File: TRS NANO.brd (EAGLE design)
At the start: 70.5 x 64.5 mm, 32 parts, among them M1 ARDUINO-NANO-3.0, Q5 BC548, Q6 BC548, Q7 BC548, Q8 BC548, T1 351, T3 351, T41 351, T42 351

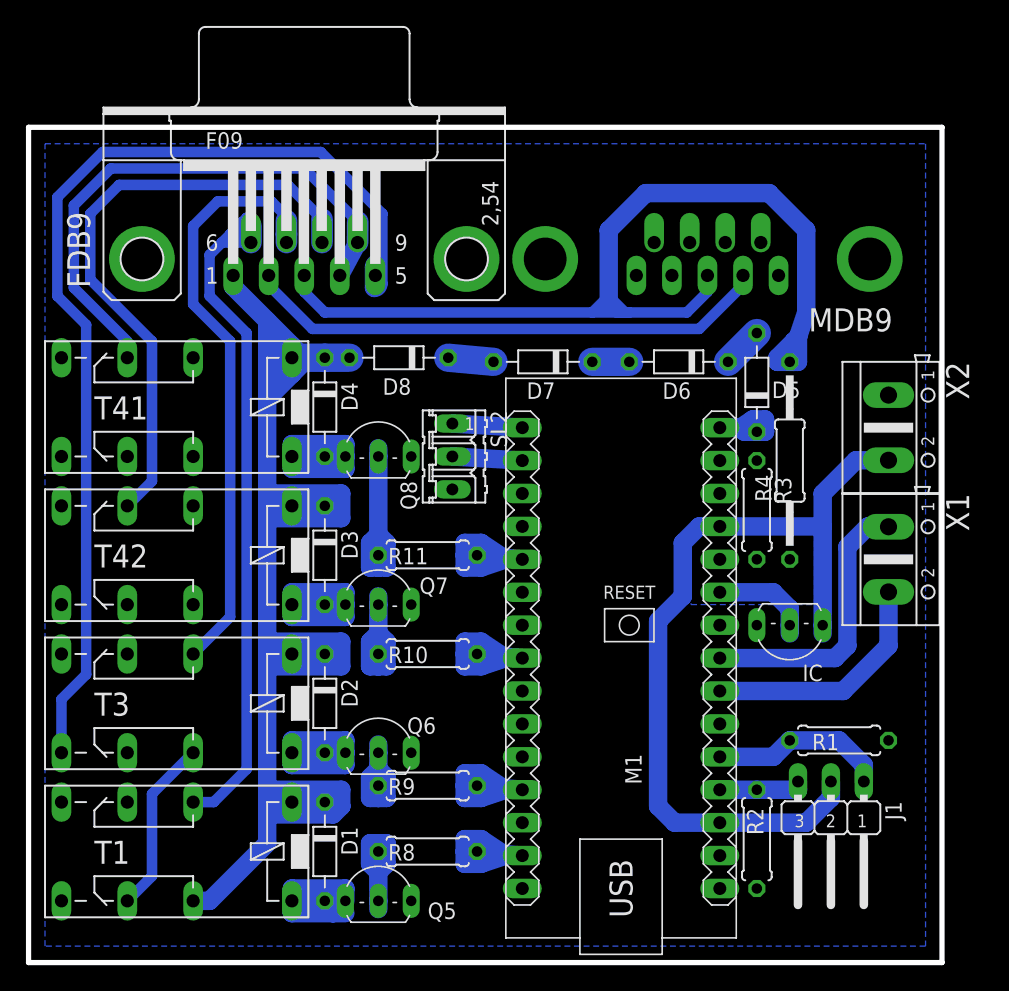
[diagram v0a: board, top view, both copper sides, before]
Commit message: Add
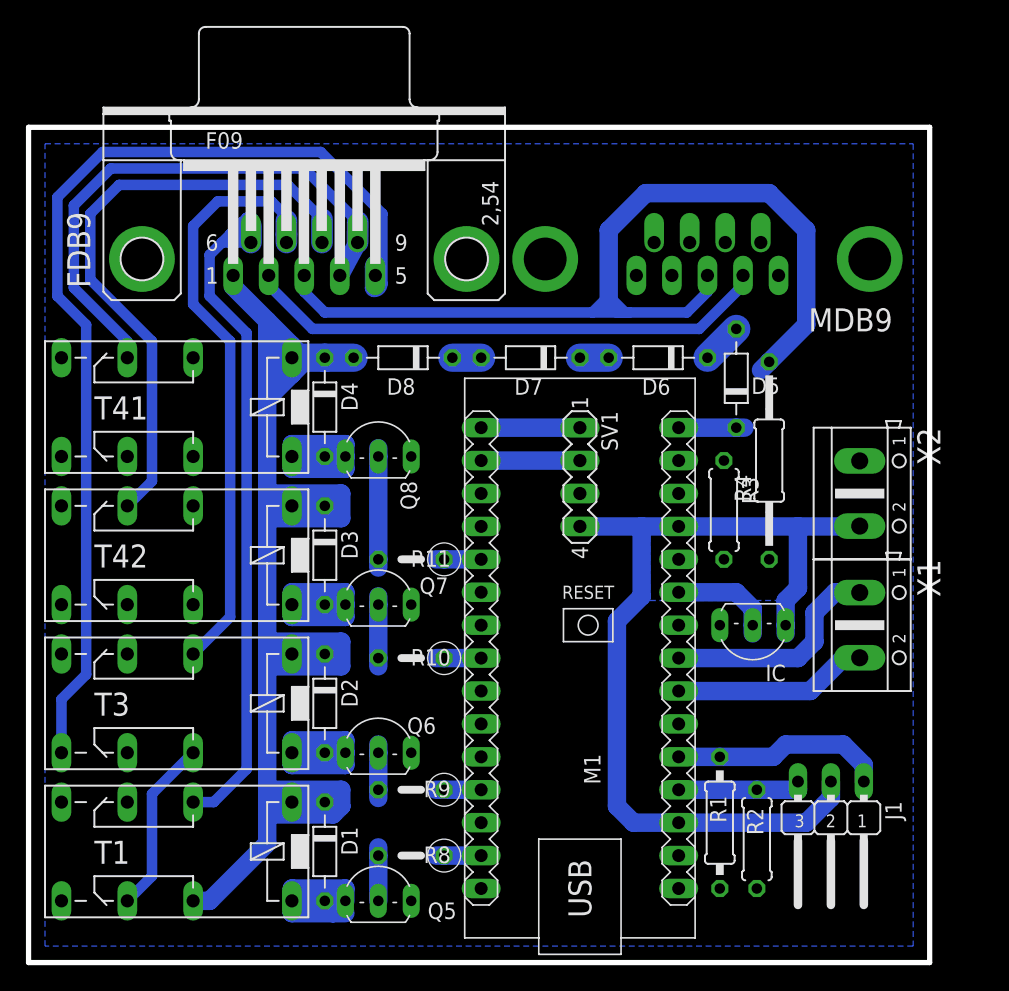
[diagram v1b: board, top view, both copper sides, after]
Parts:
- removed SL2: (no value), con-amp-quick:03P
- added SV1: (no value), con-lstb:MA04-1
- R1: device rcl:0207/7 -> rcl:0207/10
- R10, R11, R8, R9: device rcl:0207/7 -> rcl:0207/5V
- moved R1 11.2 mm to (52.1, 9.53), turned to 90 degrees
- moved X2 5.54 mm to (62.9, 34.9)
- moved X1 5.54 mm to (62.9, 24.8)
- moved M1 3.18 mm to (41.3, 22.2)
- moved IC 2.86 mm to (54.6, 23.5)
- moved R3 2.54 mm to (52.4, 33.7)
- moved D6 1.62 mm to (47.3, 45.4)
- moved D5 1.62 mm to (53.3, 43.8)
- moved R4 1.59 mm to (55.9, 37.5)
- moved R11 1.31 mm to (28.3, 29.8), turned to 180 degrees
- moved R9 1.31 mm to (28.3, 12.1), turned to 180 degrees
- moved R8 1.31 mm to (28.3, 6.99), turned to 180 degrees
- moved R10 1.31 mm to (28.3, 22.2), turned to 180 degrees
- moved D7 1.00 mm to (37.5, 45.4)
- moved D8 0.32 mm to (27.6, 45.4)
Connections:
- net +5V: now also SV1.4
- net A: now also R8.1; no longer R8.2
- net B: now also R9.1; no longer R9.2
- net C: now also R10.1; no longer R10.2
- net D: now also R11.1; no longer R11.2
- net GND: now also SV1.3; no longer SL2.3
- net N$4: now also R9.2; no longer R9.1
- net N$5: now also R10.2; no longer R10.1
- net N$6: now also R11.2; no longer R11.1
- net N$8: now also R8.2; no longer R8.1
- net RX: now also SV1.1; no longer SL2.1
- net TX: now also SV1.2; no longer SL2.2
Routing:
- net C: track 13.2 -> 3.49 mm
- net B: track 13.2 -> 3.49 mm
- net A: track 13.2 -> 3.49 mm
- net D: track 13.2 -> 3.49 mm
- net N$8: track 11.3 -> 4.13 mm
- net N$5: track 12.3 -> 5.40 mm
- net N$6: track 16.1 -> 9.21 mm
- net +5V: track 65.3 -> 71.7 mm
- net N$4: track 10.4 -> 4.13 mm
- net TRIM_A: track 21.7 -> 17.4 mm
- net TEMP: track 80.1 -> 76.0 mm
- net TRIM_B: track 18.6 -> 15.0 mm
- net A0: track 6.67 -> 9.84 mm
- net A1: track 13.7 -> 16.6 mm
- net N$7: track 7.98 -> 5.08 mm
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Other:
- board size 70.5 x 64.5 mm -> 69.5 x 64.5 mm
